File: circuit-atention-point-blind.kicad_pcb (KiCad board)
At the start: 2 copper layers, 49.3 x 36.1 mm, 26 parts, among them IC1 STM8S003F3P, P1 RS485, P2 CON 4, P3 JSN-SR04T, U1 MAX485, U2 MC34063

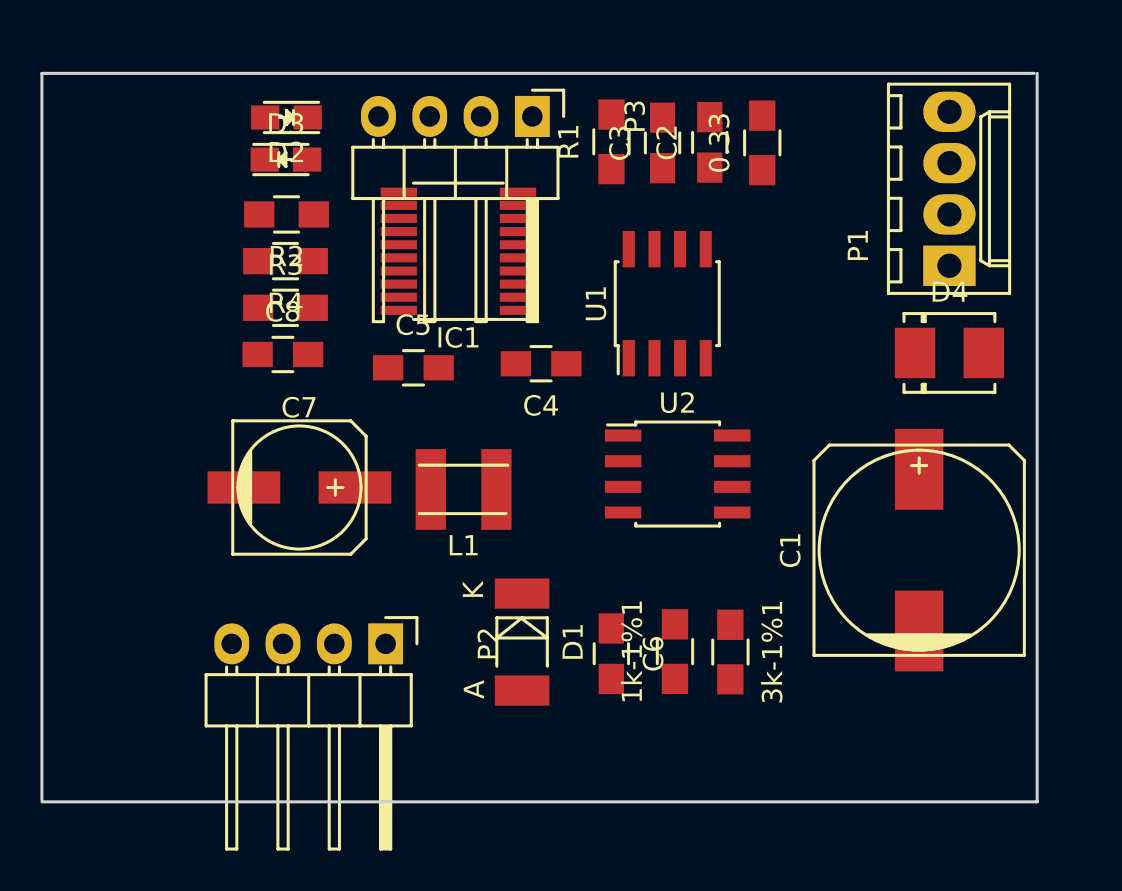
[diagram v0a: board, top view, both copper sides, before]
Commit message: backup PCB after modify 3nd
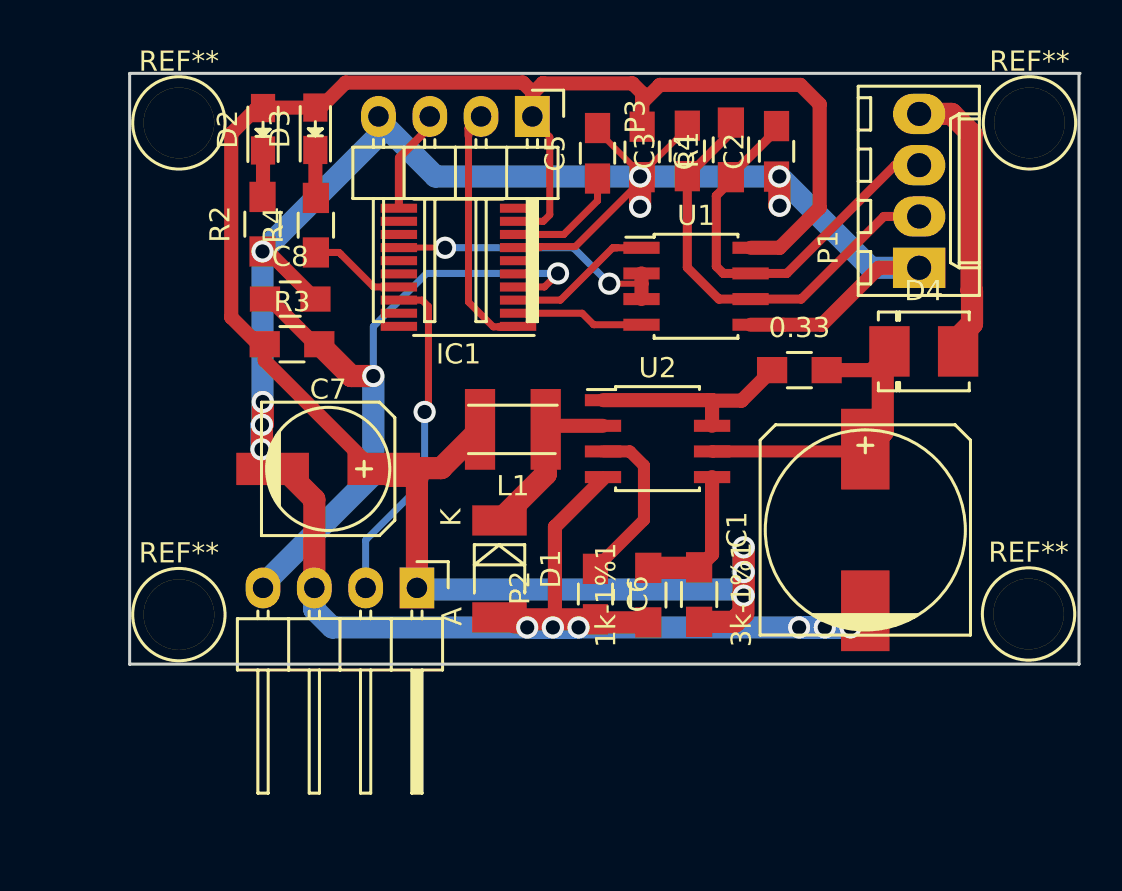
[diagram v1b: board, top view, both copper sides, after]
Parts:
- added REF**: 1pin, pad:drill-3.5mm, F.Cu at (102.1, 108.1)
- added REF**: 1pin, pad:drill-3.5mm, F.Cu at (102.0, 132.4)
- added REF**: 1pin, pad:drill-3.5mm, F.Cu at (60.0, 132.5)
- added REF**: 1pin, pad:drill-3.5mm, F.Cu at (60.0, 108.1)
- moved C5 14.0 mm to (80.7, 109.6), turned to 90 degrees
- moved C4 11.6 mm to (82.9, 109.6), turned to 270 degrees
- moved 0.33 11.4 mm to (90.7, 120.4), turned to 0 degrees
- moved R1 5.93 mm to (87.3, 109.5)
- moved L1 3.84 mm to (76.5, 123.3)
- moved D1 3.79 mm to (75.8, 130.2)
- moved C2 3.34 mm to (89.6, 109.5)
- moved 3k-1%1 3.24 mm to (85.7, 131.5)
- moved P2 3.17 mm to (71.8, 131.1)
- moved 1k-1%1 3.09 mm to (83.2, 131.5)
- moved C6 3.06 mm to (80.6, 131.4)
- moved C1 2.85 mm to (94.0, 128.3)
- moved C8 2.77 mm to (65.5, 116.8)
- moved R4 2.33 mm to (66.8, 113.2), turned to 90 degrees
- moved D3 2.11 mm to (66.7, 108.4), turned to 90 degrees
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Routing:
- net GND: track 0.00 -> 143.1 mm, vias 0 -> 13
- net +5V: track 0.00 -> 110.9 mm, vias 0 -> 3
- net /NRST: track 0.00 -> 34.6 mm, vias 0 -> 2
- net /485B: track 0.00 -> 21.9 mm
- net /485A: track 0.00 -> 20.6 mm
- net /SWIM: track 0.00 -> 17.1 mm, vias 0 -> 1
- net Net-(0.33-Pad2): track 0.00 -> 16.5 mm
- net +24V: track 0.00 -> 14.1 mm
- net /MAX485-DIR: track 0.00 -> 14.0 mm, vias 0 -> 2
- net /TRIG: track 0.00 -> 12.4 mm
- net Net-(0.33-Pad1): track 0.00 -> 10.6 mm
- net /ECHO: track 0.00 -> 10.3 mm
- net /MAX485-RX: track 0.00 -> 8.60 mm
- net Net-(C6-Pad1): track 0.00 -> 8.42 mm
- net Net-(D1-Pad1): track 0.00 -> 8.37 mm
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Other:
- board size 49.3 x 36.1 mm -> 47.1 x 29.3 mm
- net class Default: clearance 0.2 -> 0.25; trace_width 0.25 -> 0.35; via_dia 0.6 -> 1.1; via_drill 0.4 -> 0.7
- rule trace_clearance: 0.2 -> 0.25

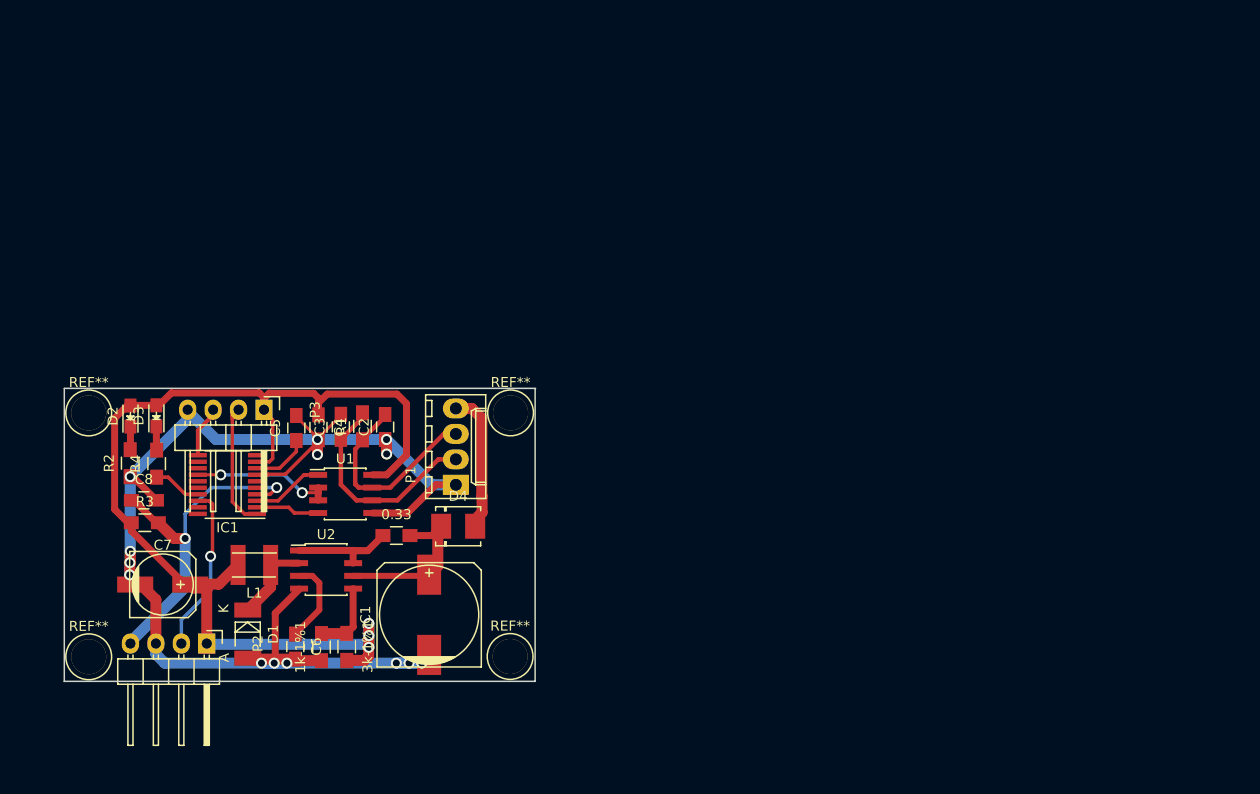
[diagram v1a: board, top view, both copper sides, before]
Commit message: finish pcb (version1)
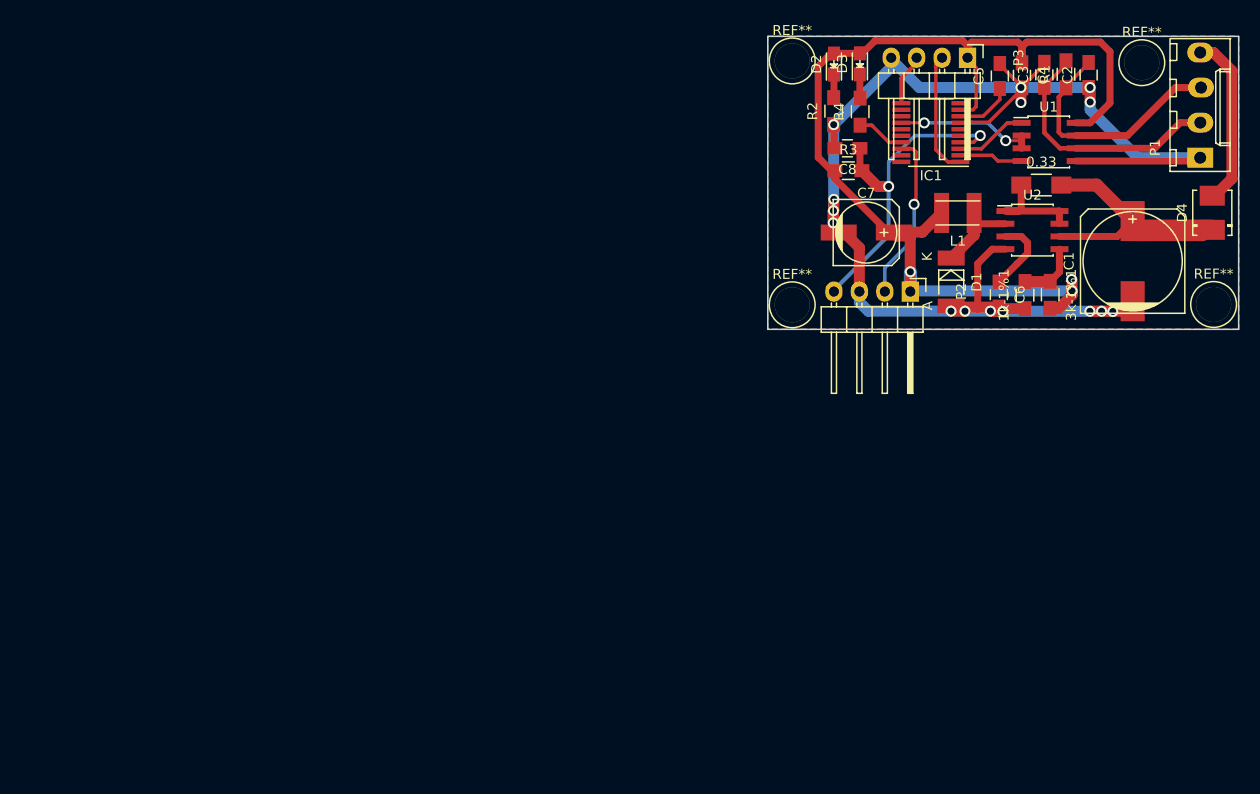
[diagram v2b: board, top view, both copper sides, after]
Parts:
- 0.33: footprint Resistors_SMD:R_0805_HandSoldering -> Resistors_SMD:R_1206_HandSoldering
- P1: footprint Connectors_Molex:Molex_KK_6410-04 -> conn:domino-big-4
- moved D4 81.5 mm to (172.1, 88.1), turned to 90 degrees
- moved P1 81.2 mm to (170.9, 82.6)
- moved C1 78.6 mm to (164.2, 93.0)
- moved C2 78.5 mm to (159.8, 74.4)
- moved C3 78.5 mm to (155.4, 74.4)
- moved C7 78.5 mm to (137.6, 90.1)
- moved D1 78.5 mm to (146.1, 95.1)
- moved L1 78.5 mm to (146.7, 88.2)
- moved R4 78.5 mm to (137.0, 78.0)
- moved 3k-1%1 78.5 mm to (156.0, 96.3)
- moved C8 78.5 mm to (135.7, 81.7), turned to 180 degrees
- moved D2 78.5 mm to (134.4, 73.3)
- moved P3 78.5 mm to (147.7, 72.7)
- moved R1 78.5 mm to (157.5, 74.3)
- moved R2 78.5 mm to (134.3, 78.0)
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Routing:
- net Net-(0.33-Pad2): track 16.5 -> 35.1 mm
- net GND: track 143.1 -> 150.7 mm, vias 13 -> 15
- net /485A: track 20.6 -> 24.5 mm
- net /485B: track 21.9 -> 25.4 mm
- net +24V: track 14.1 -> 17.3 mm
- net +5V: track 110.9 -> 109.3 mm
- net Net-(D1-Pad1): track 8.37 -> 9.72 mm
- net Net-(1k-1%1-Pad2): track 7.26 -> 6.12 mm
- net /NRST: track 34.6 -> 33.6 mm
- net Net-(C6-Pad1): track 8.42 -> 7.62 mm
- net (no net): vias 1 -> 0
- added copper zone on B.Cu, net GND
- added copper zone on F.Cu, net GND
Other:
- board size 47.1 x 29.3 mm -> 47 x 29.2 mm
- net class Default: trace_width 0.35 -> 1.3
